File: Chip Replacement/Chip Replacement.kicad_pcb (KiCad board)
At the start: 4 copper layers, 13 x 11.5 mm, 2 parts, among them J2 Conn_01x14_Socket, U1 BGA153 UFS Chip Replacement M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

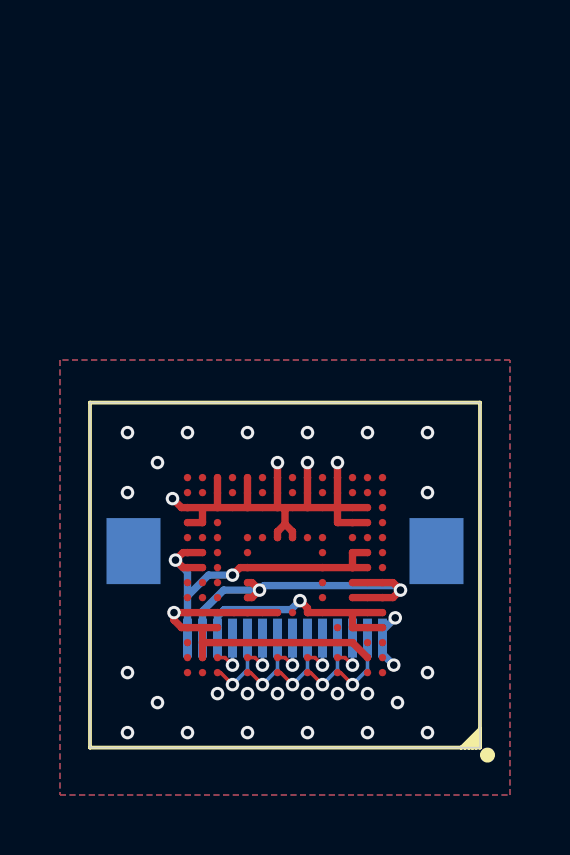
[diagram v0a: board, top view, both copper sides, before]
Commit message: V1.3 GB042 Connector
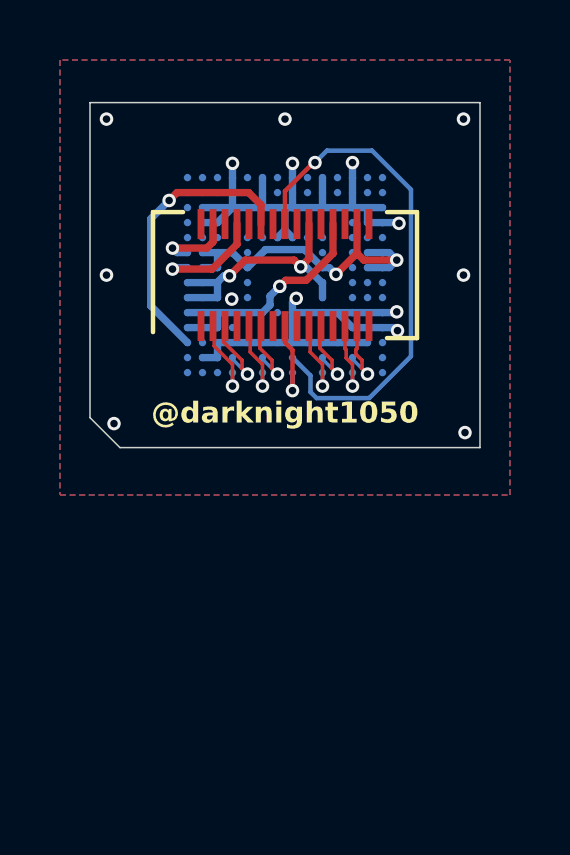
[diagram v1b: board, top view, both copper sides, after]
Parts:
- removed J2: Conn_01x14_Socket, BGA153:FPC 14 Pin 0.5P
- added J1: GB042-30S-H10, BGA153:GB042-30S-H10, F.Cu at (150.0, 90.0)
- U1: moved to B.Cu
- moved U1 10.0 mm to (150.0, 90.0), turned to 180 degrees
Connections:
- U1 pad C1: unconnected-(U1-VDDiQ-PadC1) -> /VDDiQ
- U1 pad H1: unconnected-(U1-VDDiQ2-PadH1) -> /VDDiQ2
- U1 pad J1: unconnected-(U1-VDDi-PadJ1) -> /VDDi
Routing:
- net /RST_N: track 1.50 -> 17.4 mm
- net /VDDiQ: track 0.00 -> 9.48 mm, vias 0 -> 1
- net /VDDiQ2: track 0.00 -> 3.69 mm, vias 0 -> 1
- net VCCQ2: track 12.3 -> 8.67 mm
- net /VDDi: track 0.00 -> 2.59 mm, vias 0 -> 1
- net /TX1N: track 1.50 -> 2.70 mm
- net VSS: track 31.1 -> 30.0 mm, vias 32 -> 15
- net /TX0N: track 1.50 -> 2.62 mm
- net /RX0P: track 1.50 -> 2.62 mm
- net /RX1P: track 1.50 -> 2.54 mm
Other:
- outline, holes or cut-outs redrawn
